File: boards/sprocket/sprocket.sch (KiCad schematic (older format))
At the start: 34 parts, among them J1 SPROCKET-CONN, J4 Conn_01x04_MountingPin, J5 Conn_01x04_MountingPin, J6 Conn_01x04_MountingPin, J7 Conn_01x04_MountingPin, Q1 NX7002BKR, SW1 SW_Push, SW2 SW_Push, U1 STM32G031G8U6, U2 AP2210N-3.3TRG1

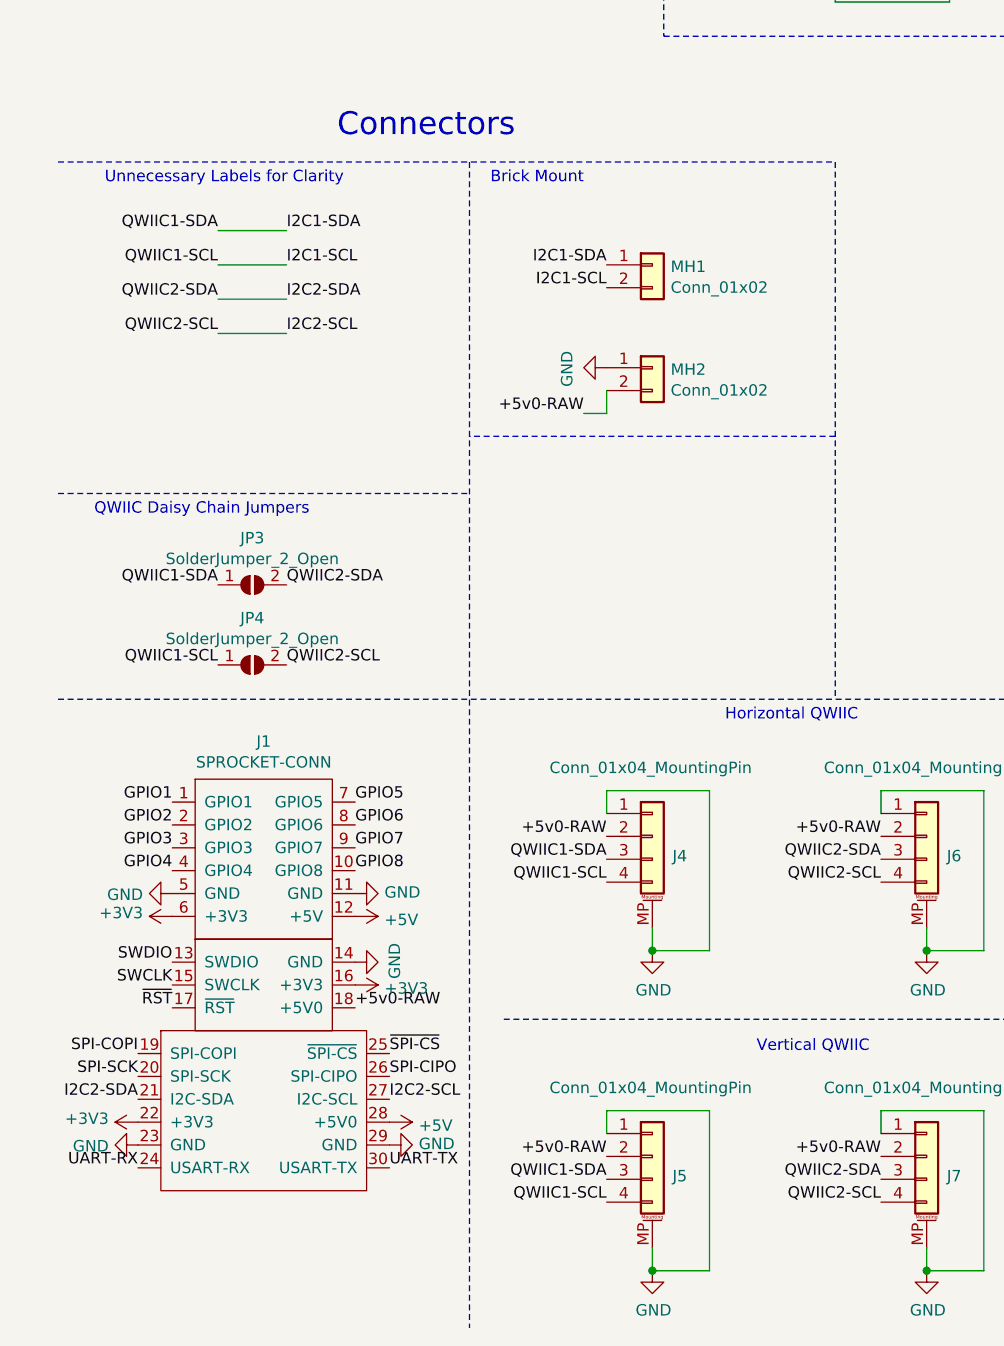
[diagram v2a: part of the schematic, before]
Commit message: Pre-order
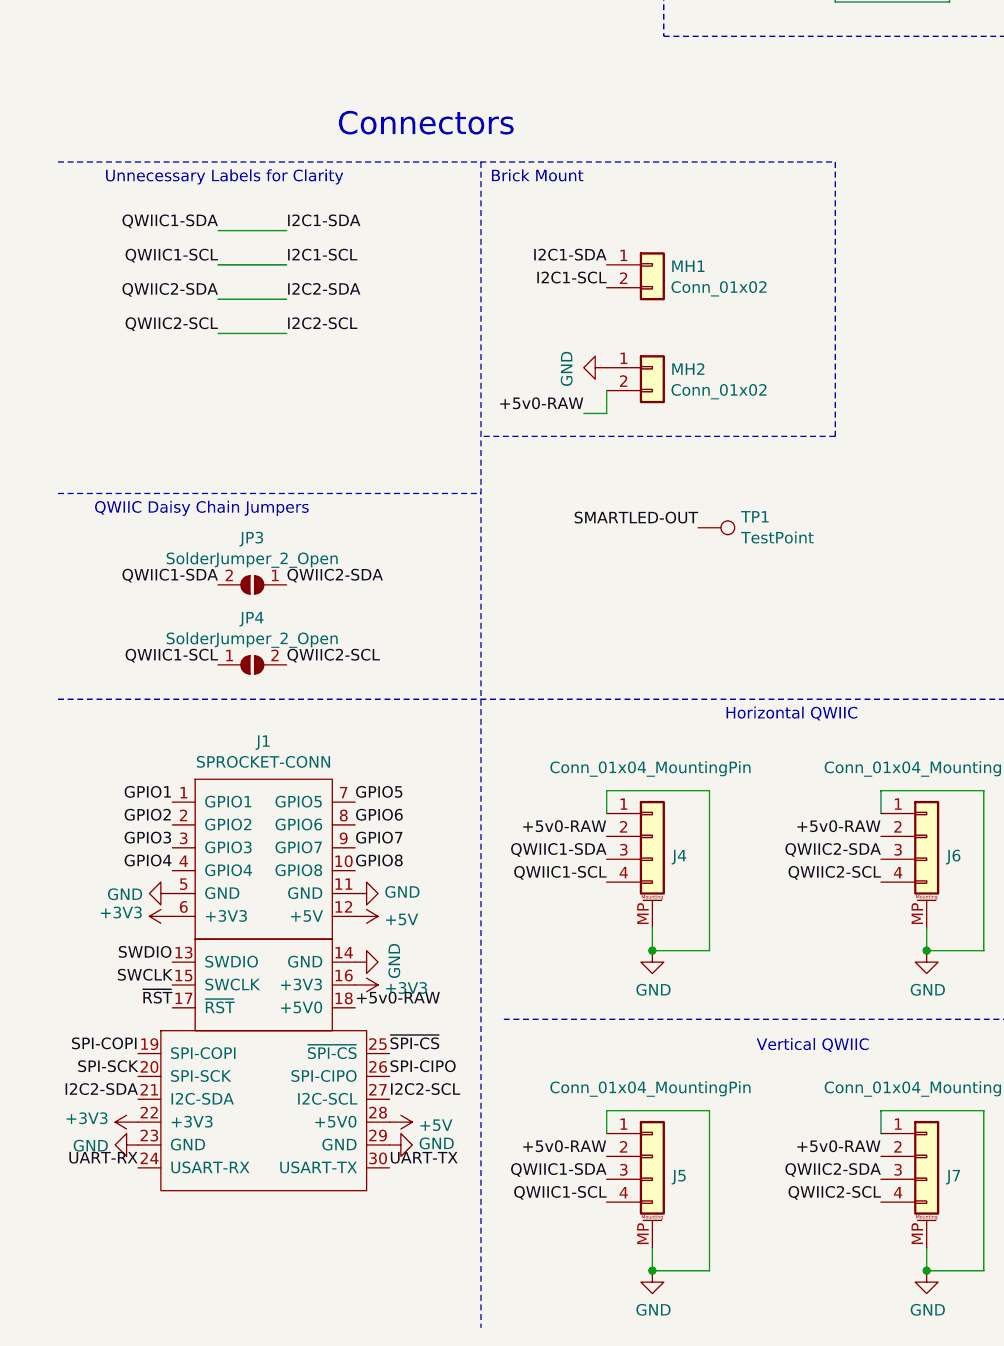
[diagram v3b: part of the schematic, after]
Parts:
- added TP1: TestPoint, TestPoint:TestPoint_Pad_D1.5mm, symbol Connector:TestPoint
- JP3, JP4: footprint Jumper:SolderJumper-2_P1.3mm_Open_TrianglePad1.0x1.5mm -> Jumper:SolderJumper-2_P1.3mm_Open_RoundedPad1.0x1.5mm
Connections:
- net I2C1-SDA: now also JP3.2 (B); no longer JP3.1 (A)
- net I2C2-SDA: now also JP3.1 (A); no longer JP3.2 (B)
- net SMARTLED-OUT: now also TP1.1
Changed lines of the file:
@@
 F 0 "JP3" H 1350 4705 50  0000 C CNN
 F 1 "SolderJumper_2_Open" H 1350 4614 50  0000 C CNN
-F 2 "Jumper:SolderJumper-2_P1.3mm_Open_TrianglePad1.0x1.5mm" H 1350 4500 50  0001 C CNN
+F 2 "Jumper:SolderJumper-2_P1.3mm_Open_RoundedPad1.0x1.5mm" H 1350 4500 50  0001 C CNN
 F 3 "~" H 1350 4500 50  0001 C CNN
 	1    1350 4500
-	1    0    0    -1
+	-1   0    0    -1
 $EndComp
 $Comp
@@
 F 0 "JP4" H 1350 5055 50  0000 C CNN
 F 1 "SolderJumper_2_Open" H 1350 4964 50  0000 C CNN
-F 2 "Jumper:SolderJumper-2_P1.3mm_Open_TrianglePad1.0x1.5mm" H 1350 4850 50  0001 C CNN
+F 2 "Jumper:SolderJumper-2_P1.3mm_Open_RoundedPad1.0x1.5mm" H 1350 4850 50  0001 C CNN
 F 3 "~" H 1350 4850 50  0001 C CNN
 	1    1350 4850
@@
 Text Label 1500 4850 0    50   ~ 0
 QWIIC2-SCL
-Wire Notes Line
-	500  4100 2300 4100
 Text Notes 1600 4200 2    50   ~ 0
 QWIIC Daisy Chain Jumpers
-Wire Notes Line
-	3900 3850 2300 3850
 Text Label 1200 2950 2    50   ~ 0
 QWIIC1-SDA
@@
 	1200 3100 1500 3100
 Wire Notes Line
-	2300 2650 2300 7750
+	2350 2650 2350 7750
 Text Notes 1750 2750 2    50   ~ 0
 Unnecessary Labels for Clarity
@@
 Brick Mount
 Wire Notes Line
-	3900 2650 3900 5000
-Wire Notes Line
 	500  2650 3900 2650
 Text Notes 2500 2550 2    100  ~ 0
@@
 Wire Wire Line
 	1500 3400 1200 3400
+Wire Notes Line
+	3900 2650 3900 3850
+Wire Notes Line
+	500  4100 2350 4100
+Wire Notes Line
+	3900 3850 2350 3850
+$Comp
+L Connector:TestPoint TP1
+U 1 1 6047197A
+P 3300 4250
+F 0 "TP1" V 3254 4438 50  0000 L CNN
+F 1 "TestPoint" V 3345 4438 50  0000 L CNN
+F 2 "TestPoint:TestPoint_Pad_D1.5mm" H 3500 4250 50  0001 C CNN
+F 3 "~" H 3500 4250 50  0001 C CNN
+	1    3300 4250
+	0    1    1    0
+$EndComp
+Text Label 3300 4250 2    50   ~ 0
+SMARTLED-OUT
 $EndSCHEMATC
